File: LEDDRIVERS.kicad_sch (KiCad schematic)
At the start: 8 parts, among them Q401 2N7002KNC, Q402 2N7002KNC

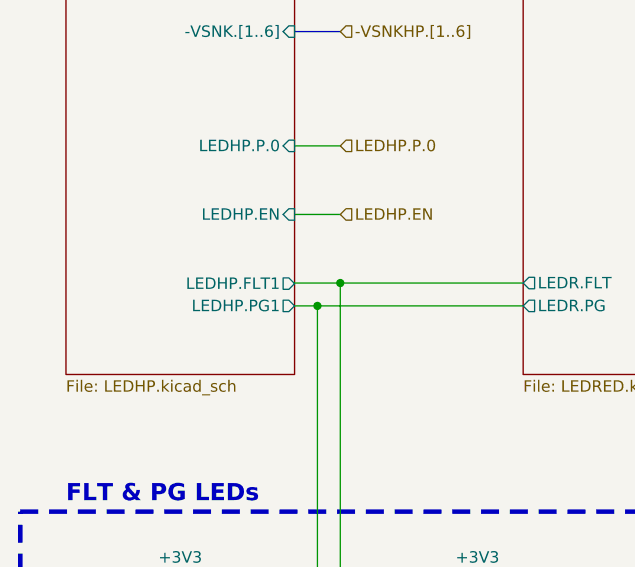
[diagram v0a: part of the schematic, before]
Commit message: Add files via upload
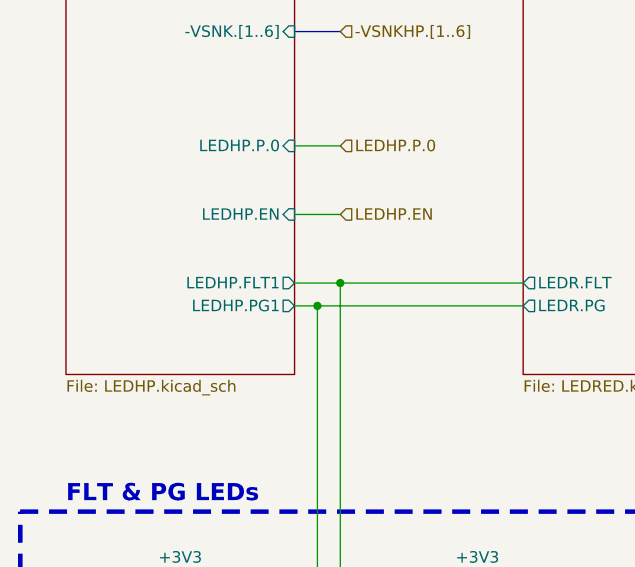
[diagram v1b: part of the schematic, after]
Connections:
- net LED RED/LEDR.FLT is gone; now on net LED CW HIGH POWER/LEDHP.FLT1: Q402.1 (G), R702.2
